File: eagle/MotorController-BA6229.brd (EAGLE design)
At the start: 35.6 x 20.3 mm, 10 parts, among them IC1 BA6229, J1 CONN-3P-3P

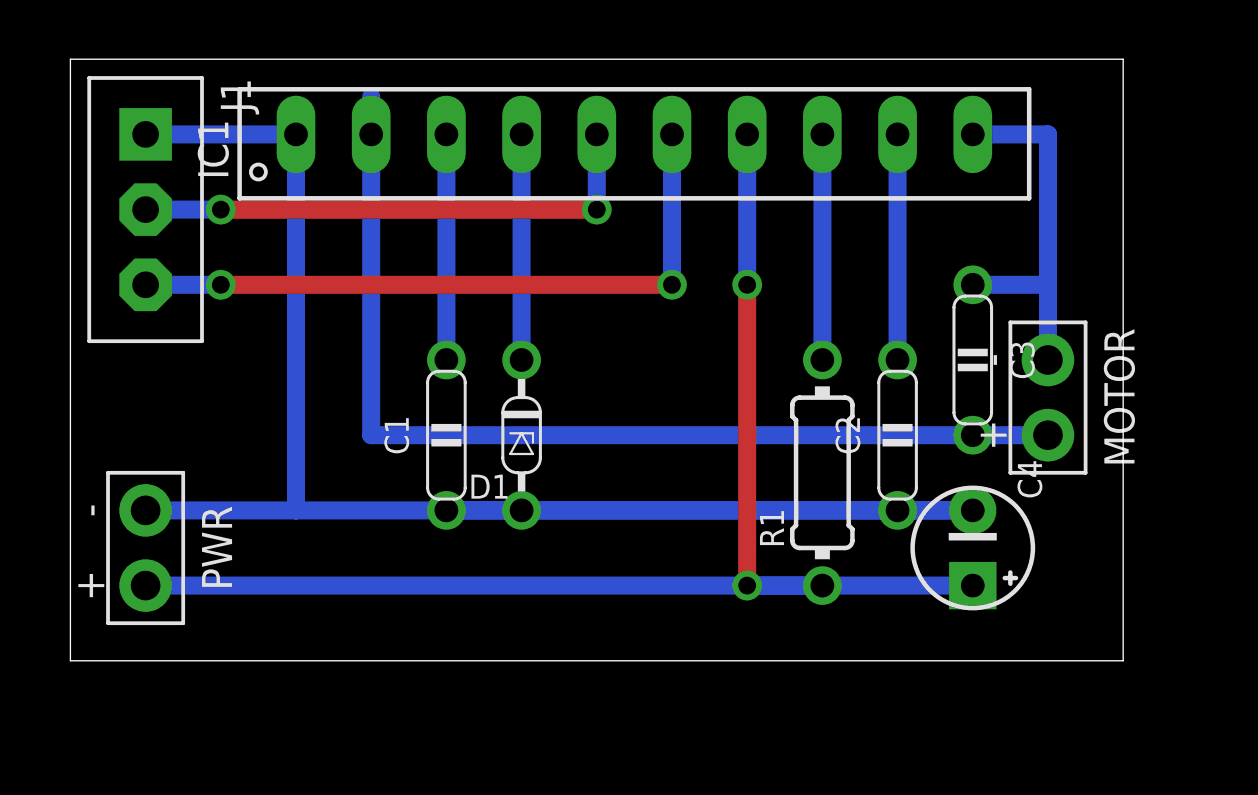
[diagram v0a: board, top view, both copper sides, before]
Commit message: ...
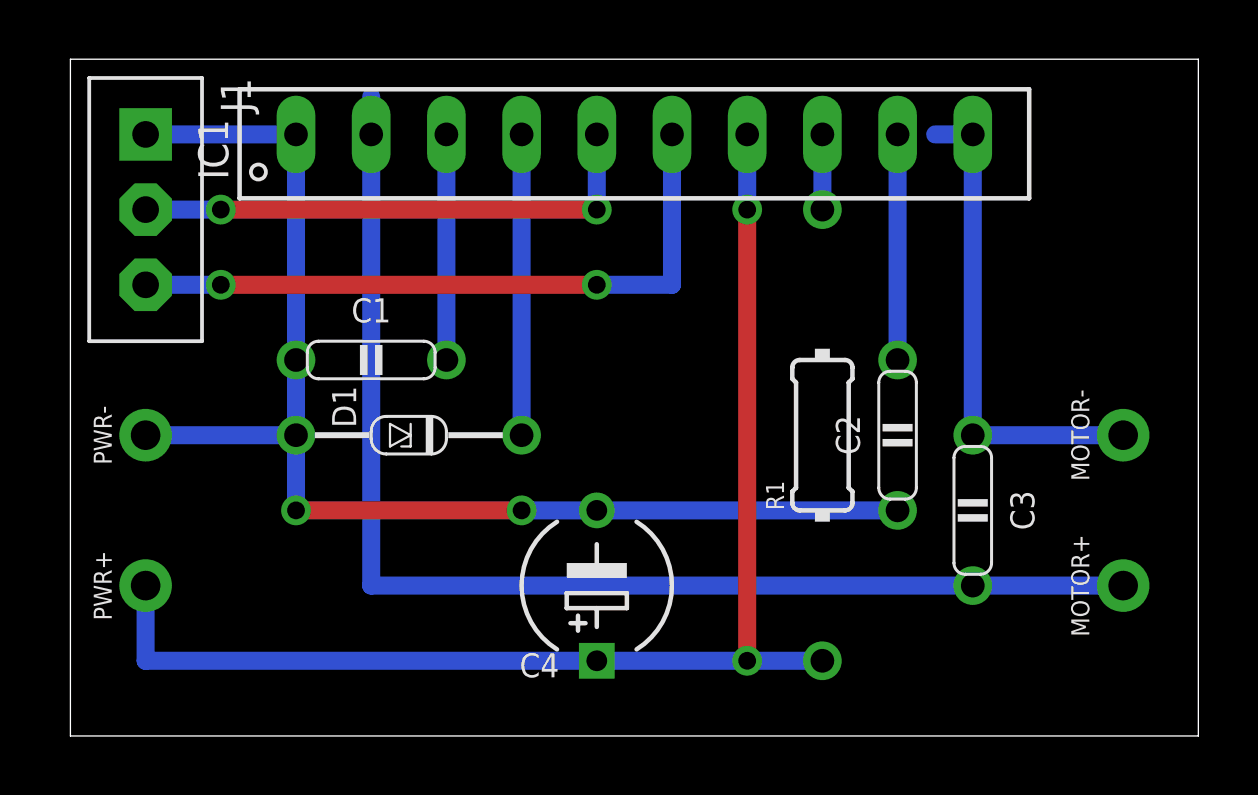
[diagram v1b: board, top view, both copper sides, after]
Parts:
- removed MOTOR, PWR: SPAD+-, pad:SPAD+-
- added MOTOR+, MOTOR-, PWR+, PWR-: SPAD, pad:SPAD
- C4: device c:E2,5-4 -> c:E5-5/V
- D1: device d:DO34Z5V -> d:DO34Z7V
- R1: device r:0204/7-V -> r:0204/15-V
- moved C4 12.8 mm to (17.8, 2.54)
- moved C3 5.08 mm to (30.5, 5.08)
- moved D1 3.81 mm to (11.4, 7.62), turned to 90 degrees
- moved C1 3.59 mm to (10.2, 10.2), turned to 0 degrees
- moved R1 1.27 mm to (25.4, 7.62)
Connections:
- net GND: now also PWR-.1; no longer PWR.1
- net N$1: now also MOTOR+.1; no longer MOTOR.2
- net N$6: now also MOTOR-.1; no longer MOTOR.1
- net VCC: now also PWR+.1; no longer PWR.2
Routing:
- net GND: track 63.5 -> 43.2 mm, vias 0 -> 2
- net N$1: track 34.3 -> 41.9 mm
- net N$8: track 7.62 -> 2.54 mm
- net N$6: track 12.7 -> 16.5 mm
- net VCC: track 45.7 -> 43.2 mm
- net N$4: track 7.62 -> 10.2 mm
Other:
- board size 35.6 x 20.3 mm -> 38.1 x 22.9 mm
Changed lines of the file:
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@@
 http://beatsdownloadg5.hatenablog.com/entry/reversible-motor-driver-circuit</description>
 <plain>
-<wire x1="0" y1="0" x2="35.56" y2="0" width="0" layer="20"/>
-<wire x1="35.56" y1="0" x2="35.56" y2="20.32" width="0" layer="20"/>
-<wire x1="35.56" y1="20.32" x2="0" y2="20.32" width="0" layer="20"/>
-<wire x1="0" y1="20.32" x2="0" y2="0" width="0" layer="20"/>
+<wire x1="0" y1="-2.54" x2="38.1" y2="-2.54" width="0" layer="20"/>
+<wire x1="38.1" y1="-2.54" x2="38.1" y2="20.32" width="0" layer="20"/>
+<wire x1="38.1" y1="20.32" x2="0" y2="20.32" width="0" layer="20"/>
+<wire x1="0" y1="20.32" x2="0" y2="-2.54" width="0" layer="20"/>
 </plain>
 <attributes>
@@
 </autorouter>
 <elements>
-<element name="C1" library="c" package="C050-020X044" value="0.1uF" x="12.7" y="7.62" rot="R90"/>
+<element name="C1" library="c" package="C050-020X044" value="0.1uF" x="10.16" y="10.16"/>
 <element name="C2" library="c" package="C050-020X044" value="0.1uF" x="27.94" y="7.62" rot="R90"/>
-<element name="C3" library="c" package="C050-020X044" value="0.33uF" x="30.48" y="10.16" rot="R270"/>
-<element name="C4" library="c" package="E2,5-4" value="100uF" x="30.48" y="3.81" rot="R180"/>
-<element name="D1" library="d" package="DO34Z5V" value="Z=4.7V" x="15.24" y="7.62" rot="R180"/>
+<element name="C3" library="c" package="C050-020X044" value="0.33uF" x="30.48" y="5.08" rot="R270"/>
+<element name="C4" library="c" package="E5-5/V" value="100uF" x="17.78" y="2.54" rot="R180"/>
+<element name="D1" library="d" package="DO34Z7V" value="Z=4.7V" x="11.43" y="7.62" rot="R90"/>
 <element name="IC1" library="ic" package="SIL10" value="BA6229" x="19.05" y="17.78" rot="R90"/>
 <element name="J1" library="pinconn" package="CONN-3P" value="CONN-3P-3P" x="2.54" y="17.78" rot="R270"/>
-<element name="MOTOR" library="pad" package="SPAD+-" value="SPAD+-" x="33.02" y="8.89" rot="R180"/>
-<element name="PWR" library="pad" package="SPAD+-" value="SPAD+-" x="2.54" y="3.81" rot="R180"/>
-<element name="R1" library="r" package="0204/7-V" value="10" x="25.4" y="6.35"/>
+<element name="R1" library="r" package="0204/15-V" value="10" x="25.4" y="7.62"/>
+<element name="MOTOR+" library="pad" package="SPAD" value="SPAD" x="35.56" y="2.54"/>
+<element name="MOTOR-" library="pad" package="SPAD" value="SPAD" x="35.56" y="7.62"/>
+<element name="PWR+" library="pad" package="SPAD" value="SPAD" x="2.54" y="2.54"/>
+<element name="PWR-" library="pad" package="SPAD" value="SPAD" x="2.54" y="7.62"/>
 </elements>
 <signals>
@@
 <contactref element="C2" pad="2"/>
 <contactref element="D1" pad="A"/>
-<contactref element="PWR" pad="1"/>
 <contactref element="C4" pad="-"/>
 <contactref element="J1" pad="1"/>
-<wire x1="2.54" y1="5.08" x2="7.62" y2="5.08" width="0.6096" layer="16"/>
-<wire x1="12.7" y1="5.08" x2="27.94" y2="5.08" width="0.6096" layer="16"/>
-<wire x1="27.94" y1="5.08" x2="30.48" y2="5.08" width="0.6096" layer="16"/>
-<wire x1="15.24" y1="5.08" x2="30.48" y2="5.08" width="0.6096" layer="16"/>
-<wire x1="15.24" y1="5.08" x2="12.7" y2="5.08" width="0.6096" layer="16"/>
 <wire x1="2.54" y1="17.78" x2="7.62" y2="17.78" width="0.6096" layer="16"/>
-<wire x1="12.7" y1="5.08" x2="7.62" y2="5.08" width="0.6096" layer="16"/>
-<wire x1="7.62" y1="5.08" x2="7.62" y2="17.78" width="0.6096" layer="16"/>
+<wire x1="7.62" y1="10.16" x2="7.62" y2="7.62" width="0.6096" layer="16"/>
+<contactref element="PWR-" pad="1"/>
+<wire x1="7.62" y1="10.16" x2="7.62" y2="17.78" width="0.6096" layer="16"/>
+<wire x1="2.54" y1="7.62" x2="7.62" y2="7.62" width="0.6096" layer="16"/>
+<wire x1="17.78" y1="5.08" x2="15.24" y2="5.08" width="0.6096" layer="16"/>
+<via x="15.24" y="5.08" extent="1-16" drill="0.6" shape="square"/>
+<wire x1="15.24" y1="5.08" x2="7.62" y2="5.08" width="0.6096" layer="1"/>
+<via x="7.62" y="5.08" extent="1-16" drill="0.6" shape="square"/>
+<wire x1="7.62" y1="5.08" x2="7.62" y2="7.62" width="0.6096" layer="16"/>
+<wire x1="17.78" y1="5.08" x2="27.94" y2="5.08" width="0.6096" layer="16"/>
 </signal>
 <signal name="N$2">
@@
 <contactref element="IC1" pad="4"/>
 <contactref element="D1" pad="C"/>
-<wire x1="15.24" y1="17.78" x2="15.24" y2="10.16" width="0.6096" layer="16"/>
+<wire x1="15.24" y1="17.78" x2="15.24" y2="7.62" width="0.6096" layer="16"/>
 </signal>
 <signal name="N$1">
 <contactref element="IC1" pad="2"/>
-<contactref element="MOTOR" pad="2"/>
 <contactref element="C3" pad="1"/>
-<wire x1="33.02" y1="7.62" x2="30.48" y2="7.62" width="0.6096" layer="16"/>
-<wire x1="30.48" y1="7.62" x2="10.16" y2="7.62" width="0.6096" layer="16"/>
-<wire x1="10.16" y1="7.62" x2="10.16" y2="17.78" width="0.6096" layer="16"/>
+<wire x1="30.48" y1="2.54" x2="10.16" y2="2.54" width="0.6096" layer="16"/>
+<wire x1="10.16" y1="2.54" x2="10.16" y2="17.78" width="0.6096" layer="16"/>
 <wire x1="10.16" y1="19.05" x2="10.16" y2="17.78" width="0.6096" layer="16"/>
+<contactref element="MOTOR+" pad="1"/>
+<wire x1="35.56" y1="2.54" x2="30.48" y2="2.54" width="0.6096" layer="16"/>
 </signal>
 <signal name="N$6">
-<contactref element="MOTOR" pad="1"/>
 <contactref element="IC1" pad="10"/>
 <contactref element="C3" pad="2"/>
-<wire x1="33.02" y1="10.16" x2="33.02" y2="12.7" width="0.6096" layer="16"/>
-<wire x1="30.48" y1="17.78" x2="33.02" y2="17.78" width="0.6096" layer="16"/>
-<wire x1="33.02" y1="17.78" x2="33.02" y2="12.7" width="0.6096" layer="16"/>
-<wire x1="33.02" y1="12.7" x2="30.48" y2="12.7" width="0.6096" layer="16"/>
+<contactref element="MOTOR-" pad="1"/>
+<wire x1="35.56" y1="7.62" x2="30.48" y2="7.62" width="0.6096" layer="16"/>
+<wire x1="30.48" y1="7.62" x2="30.48" y2="17.78" width="0.6096" layer="16"/>
+<wire x1="30.48" y1="17.78" x2="29.21" y2="17.78" width="0.6096" layer="16"/>
 </signal>
 <signal name="N$8">
 <contactref element="IC1" pad="8"/>
 <contactref element="R1" pad="1"/>
-<wire x1="25.4" y1="10.16" x2="25.4" y2="17.78" width="0.6096" layer="16"/>
+<wire x1="25.4" y1="15.24" x2="25.4" y2="17.78" width="0.6096" layer="16"/>
 </signal>
 <signal name="VCC">
 <contactref element="IC1" pad="7"/>
 <contactref element="R1" pad="2"/>
-<contactref element="PWR" pad="2"/>
 <contactref element="C4" pad="+"/>
-<wire x1="22.86" y1="17.78" x2="22.86" y2="12.7" width="0.6096" layer="16"/>
-<wire x1="22.86" y1="12.7" x2="22.86" y2="2.54" width="0.6096" layer="1"/>
-<wire x1="22.86" y1="2.54" x2="2.54" y2="2.54" width="0.6096" layer="16"/>
-<via x="22.86" y="12.7" extent="1-16" drill="0.6" shape="square"/>
-<via x="22.86" y="2.54" extent="1-16" drill="0.6" shape="square"/>
-<wire x1="22.86" y1="2.54" x2="25.4" y2="2.54" width="0.6096" layer="16"/>
-<wire x1="22.86" y1="2.54" x2="30.48" y2="2.54" width="0.6096" layer="16"/>
+<wire x1="22.86" y1="17.78" x2="22.86" y2="15.24" width="0.6096" layer="16"/>
+<wire x1="22.86" y1="15.24" x2="22.86" y2="0" width="0.6096" layer="1"/>
+<via x="22.86" y="15.24" extent="1-16" drill="0.6" shape="square"/>
+<via x="22.86" y="0" extent="1-16" drill="0.6" shape="square"/>
+<wire x1="22.86" y1="0" x2="25.4" y2="0" width="0.6096" layer="16"/>
+<wire x1="22.86" y1="0" x2="17.78" y2="0" width="0.6096" layer="16"/>
+<contactref element="PWR+" pad="1"/>
+<wire x1="17.78" y1="0" x2="2.54" y2="0" width="0.6096" layer="16"/>
+<wire x1="2.54" y1="0" x2="2.54" y2="2.54" width="0.6096" layer="16"/>
 </signal>
 <signal name="N$5">
@@
 <wire x1="2.54" y1="12.7" x2="5.08" y2="12.7" width="0.6096" layer="16"/>
 <via x="5.08" y="12.7" extent="1-16" drill="0.6" shape="square"/>
-<wire x1="5.08" y1="12.7" x2="20.32" y2="12.7" width="0.6096" layer="1"/>
-<via x="20.32" y="12.7" extent="1-16" drill="0.6" shape="square"/>
-<wire x1="20.32" y1="12.7" x2="20.32" y2="17.78" width="0.6096" layer="16"/>
+<wire x1="5.08" y1="12.7" x2="17.78" y2="12.7" width="0.6096" layer="1"/>
+<via x="17.78" y="12.7" extent="1-16" drill="0.6" shape="square"/>
+<wire x1="17.78" y1="12.7" x2="20.32" y2="12.7" width="0.6096" layer="16"/>
+<wire x1="20.32" y1="12.7" x2="20.32" y2="13.97" width="0.6096" layer="16"/>
+<wire x1="20.32" y1="13.97" x2="20.32" y2="17.78" width="0.6096" layer="16"/>
 </signal>
 </signals>
